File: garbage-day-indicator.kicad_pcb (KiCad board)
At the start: 2 copper layers, 46 x 63 mm, 18 parts, among them J1 Conn_01x16, J2 Conn_01x16

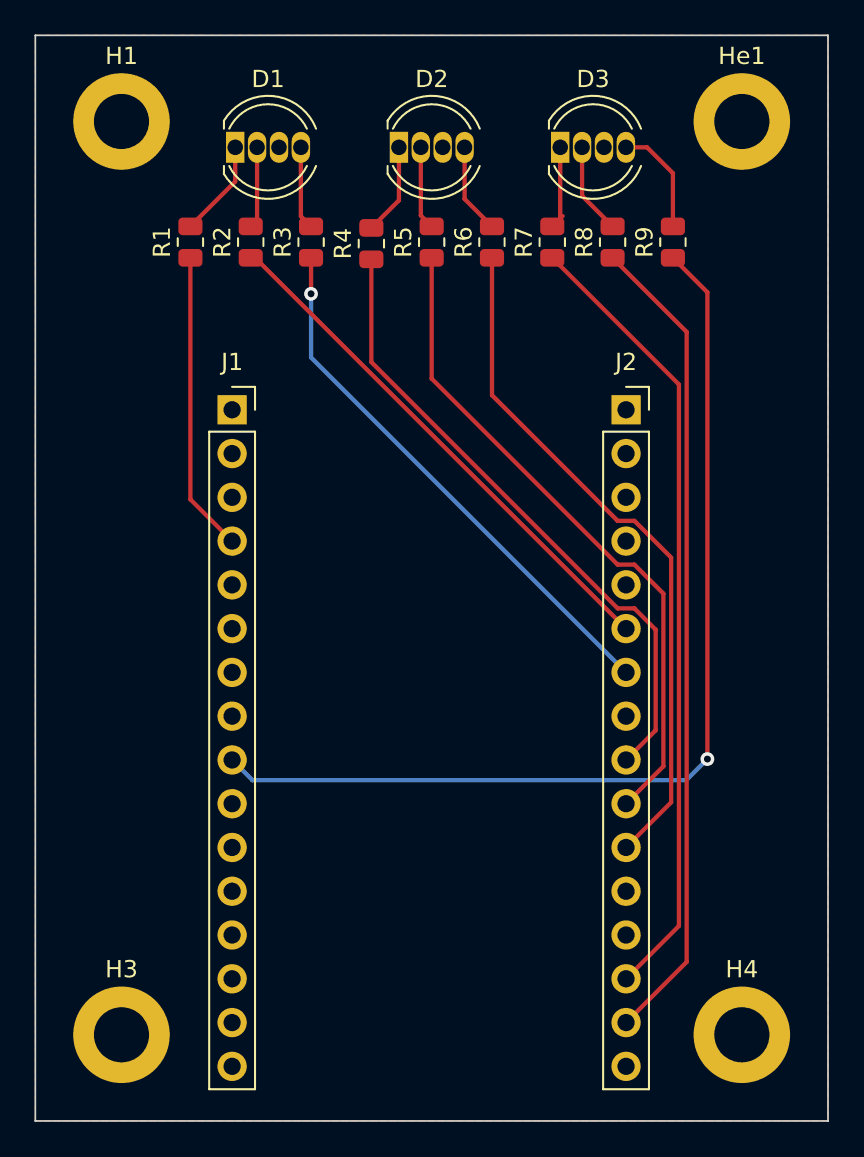
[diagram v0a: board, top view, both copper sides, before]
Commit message: Improve pcb layout
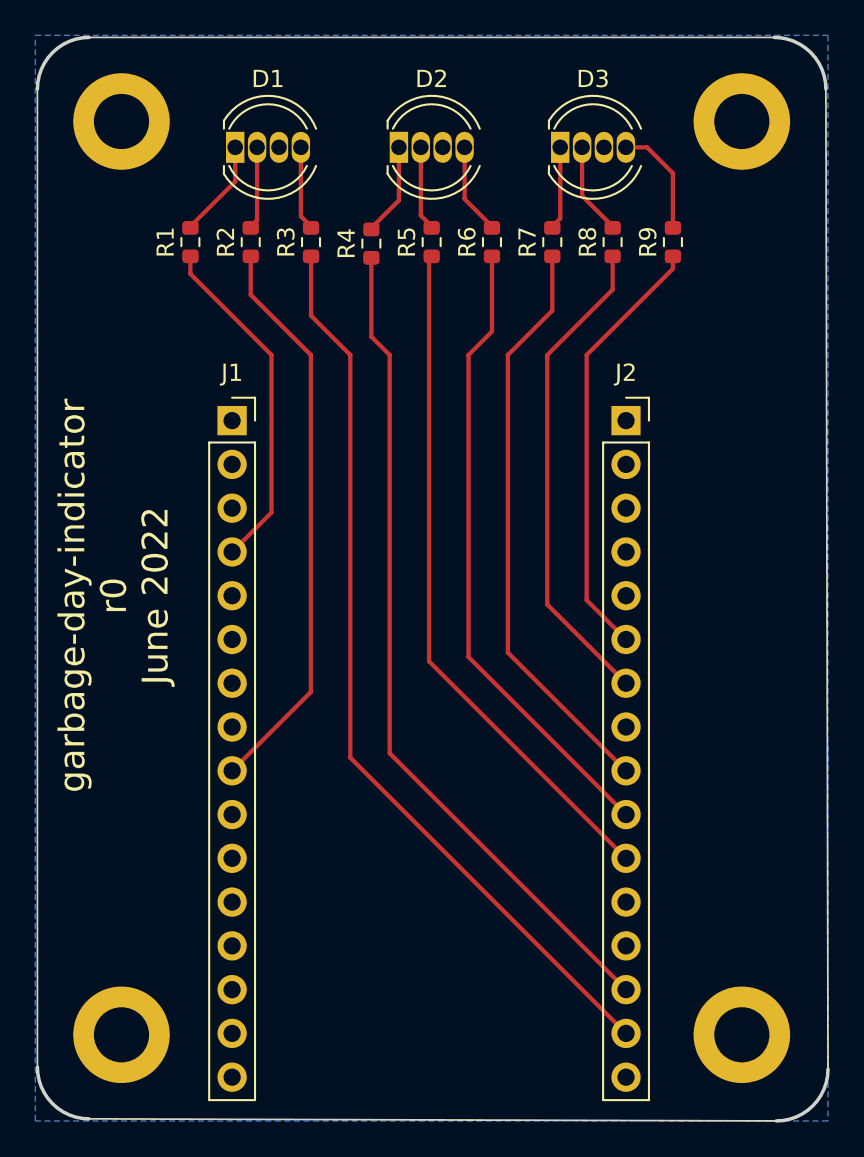
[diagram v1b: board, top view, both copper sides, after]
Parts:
- R1, R2, R3, R4, R5, R6, R7, R8, R9: footprint Resistor_SMD:R_0805_2012Metric -> Resistor_SMD:R_0603_1608Metric
- moved J1 0.63 mm to (107.4, 80.4)
- moved J2 0.63 mm to (130.3, 80.4)
- renumbered He1 to H2
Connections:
- J1 pad 9: /B3 -> /G1
- J2 pad 10: /G2 -> /B2
- J2 pad 11: /B2 -> /G2
- J2 pad 14: /R3 -> /R2
- J2 pad 15: /G3 -> /B1
- J2 pad 6: /G1 -> /B3
- J2 pad 7: /B1 -> /G3
- J2 pad 9: /R2 -> /R3
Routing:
- net /B3: track 58.5 -> 25.2 mm, vias 1 -> 0
- net /B1: track 31.6 -> 52.6 mm, vias 1 -> 0
- net /G3: track 47.6 -> 28.2 mm
- net /R3: track 46.2 -> 33.7 mm
- net /R2: track 37.2 -> 48.5 mm
- net /B2: track 40.2 -> 36.7 mm
- net /R1: track 17.4 -> 20.0 mm
- net /G1: track 30.7 -> 33.2 mm
- net /G2: track 38.7 -> 39.6 mm
- net Net-(D3-Pad1): track 5.63 -> 4.78 mm
- added copper zone on B.Cu, net GND
- removed copper zone on F.Cu, net GND
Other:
- board size 46 x 63 mm -> 45.9 x 62.9 mm
- board text added: "garbage-day-indicator r0 June 2022"
